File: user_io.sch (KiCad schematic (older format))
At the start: 39 parts, among them J3 Conn_02x05_Odd_Even, J4 Conn_01x06_Male, J5 Conn_01x05_Male, J6 Conn_01x04_Male, J7 Conn_01x09_Male, J8 Conn_01x04_Male, SW1 SW_Push_Dual, SW2 SW_Push_Dual, SW3 SW_Push_Dual, U3 STM32F051R8T6, U4 CAT24C256, Y1 8MHz

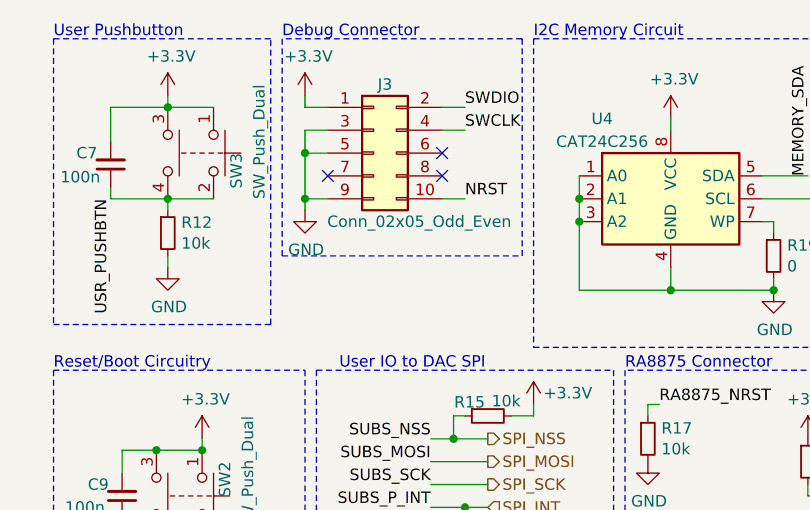
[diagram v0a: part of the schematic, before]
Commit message: Huge progress on routing
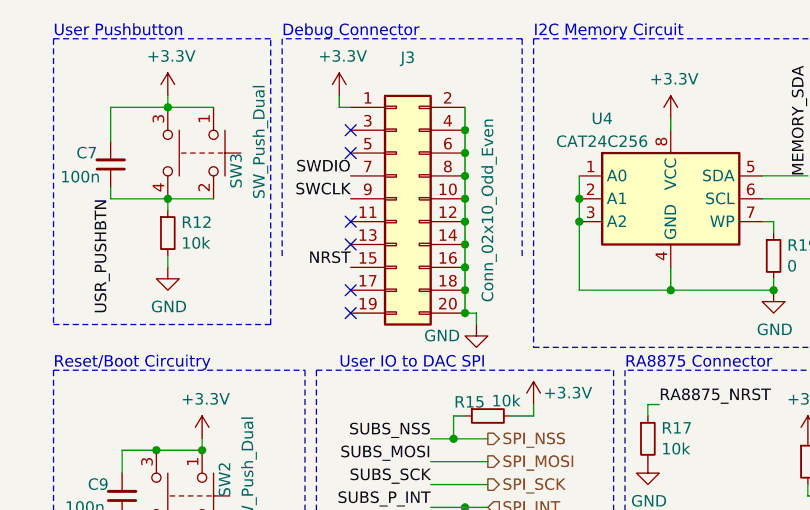
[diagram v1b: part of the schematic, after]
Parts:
- removed J3: Conn_02x05_Odd_Even, Connector_PinHeader_2.54mm:PinHeader_2x05_P2.54mm_Vertical, symbol Connector_Generic:Conn_02x05_Odd_Even
- added J3: Conn_02x10_Odd_Even, Connector_PinHeader_1.27mm:PinHeader_2x10_P1.27mm_Vertical, symbol Connector_Generic:Conn_02x10_Odd_Even
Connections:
- net +3V3: now also J3.1 (Pin_1)
- net GND: now also J3.10 (Pin_10), J3.12 (Pin_12), J3.14 (Pin_14), J3.16 (Pin_16), J3.18 (Pin_18), J3.2 (Pin_2), J3.20 (Pin_20), J3.4 (Pin_4), J3.6 (Pin_6), J3.8 (Pin_8)
- net NRST: now also J3.15 (Pin_15)
- net SWCLK: now also J3.9 (Pin_9)
- net SWDIO: now also J3.7 (Pin_7)
- no-connect marks 38 -> 41
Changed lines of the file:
@@
 	2800 2600 2650 2600
-$Comp
-L Connector_Generic:Conn_02x05_Odd_Even J3
-U 1 1 61020F75
-P 6800 1200
-F 0 "J3" H 6850 1500 50  0000 C CNN
-F 1 "Conn_02x05_Odd_Even" H 7000 900 50  0000 C CNN
-F 2 "Connector_PinHeader_2.54mm:PinHeader_2x05_P2.54mm_Vertical" H 6800 1200 50  0001 C CNN
-F 3 "~" H 6800 1200 50  0001 C CNN
-F 4 "STLink header for programming/debugging" H 6800 1200 50  0001 C CNN "Description"
-	1    6800 1200
-	1    0    0    -1
-$EndComp
 $Comp
 L power:GND #PWR028
 U 1 1 6102234A
-P 6500 1450
-F 0 "#PWR028" H 6500 1200 50  0001 C CNN
-F 1 "GND" H 6505 1277 50  0000 C CNN
-F 2 "" H 6500 1450 50  0001 C CNN
-F 3 "" H 6500 1450 50  0001 C CNN
-	1    6500 1450
-	1    0    0    -1
-$EndComp
-Wire Wire Line
-	6500 1450 6500 1400
-Wire Wire Line
-	6500 1400 6600 1400
-Wire Wire Line
-	6500 1400 6500 1200
-Wire Wire Line
-	6500 1200 6600 1200
-Connection ~ 6500 1400
-Wire Wire Line
-	6500 1200 6500 1100
-Wire Wire Line
-	6500 1100 6600 1100
-Connection ~ 6500 1200
+P 7250 1950
+F 0 "#PWR028" H 7250 1700 50  0001 C CNN
+F 1 "GND" H 7100 1900 50  0000 C CNN
+F 2 "" H 7250 1950 50  0001 C CNN
+F 3 "" H 7250 1950 50  0001 C CNN
+	1    7250 1950
+	1    0    0    -1
+$EndComp
 $Comp
 L power:+3.3V #PWR027
 U 1 1 61024D4E
-P 6500 950
-F 0 "#PWR027" H 6500 800 50  0001 C CNN
-F 1 "+3.3V" H 6515 1123 50  0000 C CNN
-F 2 "" H 6500 950 50  0001 C CNN
-F 3 "" H 6500 950 50  0001 C CNN
-	1    6500 950
-	1    0    0    -1
-$EndComp
-Wire Wire Line
-	6500 950  6500 1000
-Wire Wire Line
-	6500 1000 6600 1000
-NoConn ~ 6600 1300
-NoConn ~ 7100 1300
-NoConn ~ 7100 1200
+P 6650 950
+F 0 "#PWR027" H 6650 800 50  0001 C CNN
+F 1 "+3.3V" H 6665 1123 50  0000 C CNN
+F 2 "" H 6650 950 50  0001 C CNN
+F 3 "" H 6650 950 50  0001 C CNN
+	1    6650 950
+	1    0    0    -1
+$EndComp
 Text Label 1300 2600 2    50   ~ 0
 NRST
 Wire Wire Line
 	1300 2600 1450 2600
-Text Label 7200 1400 0    50   ~ 0
+Text Label 6700 1700 2    50   ~ 0
 NRST
-Wire Wire Line
-	7200 1400 7100 1400
-Text Label 7200 1000 0    50   ~ 0
+Text Label 6700 1300 2    50   ~ 0
 SWDIO
-Text Label 7200 1100 0    50   ~ 0
+Text Label 6700 1400 2    50   ~ 0
 SWCLK
-Wire Wire Line
-	7200 1100 7100 1100
-Wire Wire Line
-	7100 1000 7200 1000
 $Comp
 L Device:C_Small C10
@@
 Text Notes 5400 2150 0    50   ~ 0
 Reset/Boot Circuitry
-Wire Notes Line
-	6400 1650 7450 1650
 Wire Notes Line
 	7450 1650 7450 700
@@
 Wire Wire Line
 	9450 2600 10050 2600
+$Comp
+L Connector_Generic:Conn_02x10_Odd_Even J3
+U 1 1 606691DA
+P 6900 1400
+F 0 "J3" H 6950 2017 50  0000 C CNN
+F 1 "Conn_02x10_Odd_Even" V 7300 1350 50  0000 C CNN
+F 2 "Connector_PinHeader_1.27mm:PinHeader_2x10_P1.27mm_Vertical" H 6900 1400 50  0001 C CNN
+F 3 "~" H 6900 1400 50  0001 C CNN
+	1    6900 1400
+	1    0    0    -1
+$EndComp
+NoConn ~ 6700 1500
+NoConn ~ 6700 1600
+NoConn ~ 6700 1800
+NoConn ~ 6700 1900
+NoConn ~ 6700 1100
+NoConn ~ 6700 1200
+Wire Wire Line
+	6650 950  6650 1000
+Wire Wire Line
+	6650 1000 6700 1000
+Wire Wire Line
+	7250 1950 7250 1900
+Wire Wire Line
+	7250 1900 7200 1900
+Wire Wire Line
+	7200 1900 7200 1800
+Connection ~ 7200 1900
+Connection ~ 7200 1100
+Wire Wire Line
+	7200 1100 7200 1000
+Connection ~ 7200 1200
+Wire Wire Line
+	7200 1200 7200 1100
+Connection ~ 7200 1300
+Wire Wire Line
+	7200 1300 7200 1200
+Connection ~ 7200 1400
+Wire Wire Line
+	7200 1400 7200 1300
+Connection ~ 7200 1500
+Wire Wire Line
+	7200 1500 7200 1400
+Connection ~ 7200 1600
+Wire Wire Line
+	7200 1600 7200 1500
+Connection ~ 7200 1700
+Wire Wire Line
+	7200 1700 7200 1600
+Connection ~ 7200 1800
+Wire Wire Line
+	7200 1800 7200 1700
 $EndSCHEMATC
